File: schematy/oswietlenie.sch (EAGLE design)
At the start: 9 parts, among them U1 V_REG_317SINK

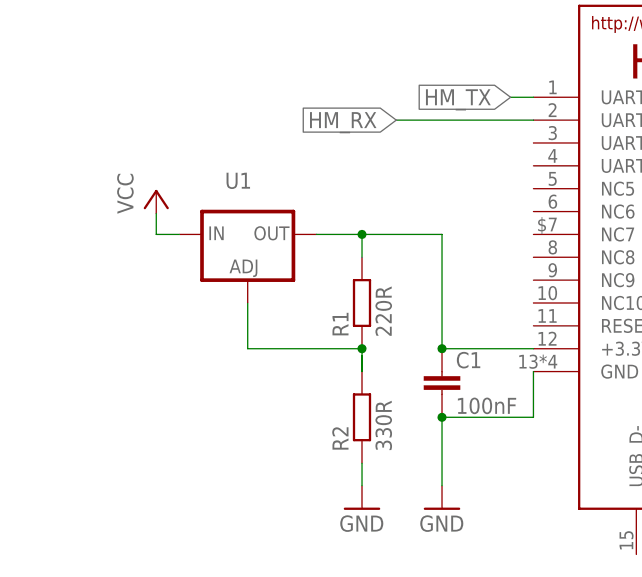
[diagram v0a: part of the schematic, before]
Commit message: update`
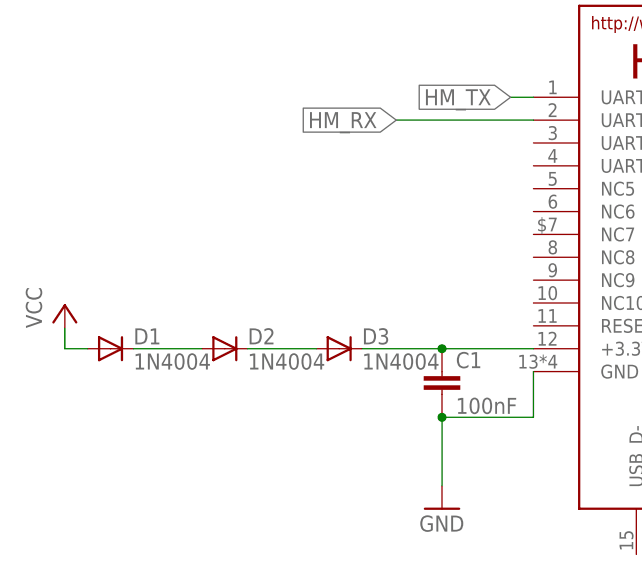
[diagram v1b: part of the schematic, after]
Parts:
- removed R1: 220R, rcl:R-EU_0204/5
- removed R2: 330R, rcl:R-EU_0204/5
- removed U1: V_REG_317SINK, SparkFun-IC-Power:V_REG_317SINK
- added D1, D2, D3: 1N4004, diode:1N4004
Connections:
- new net N$1: D1.C, D2.A
- net GND: no longer R2.1
- net N$5: now also D3.C; no longer R1.2, U1.OUT
- net N$6: now also D2.C, D3.A; no longer R1.1, R2.2, U1.ADJ
- net VCC: now also D1.A; no longer U1.IN
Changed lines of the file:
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@@
 <part name="GND5" library="supply1" library_urn="urn:adsk.eagle:library:371" deviceset="GND" device=""/>
 <part name="P+5" library="supply1" library_urn="urn:adsk.eagle:library:371" deviceset="+5V" device=""/>
-<part name="R1" library="rcl" library_urn="urn:adsk.eagle:library:334" deviceset="R-EU_" device="0204/5" package3d_urn="urn:adsk.eagle:package:23488/1" value="220R"/>
-<part name="R2" library="rcl" library_urn="urn:adsk.eagle:library:334" deviceset="R-EU_" device="0204/5" package3d_urn="urn:adsk.eagle:package:23488/1" value="330R"/>
-<part name="GND2" library="supply1" library_urn="urn:adsk.eagle:library:371" deviceset="GND" device=""/>
 <part name="~220V" library="jumper" library_urn="urn:adsk.eagle:library:252" deviceset="JP1E" device="" package3d_urn="urn:adsk.eagle:package:15455/1"/>
-<part name="U1" library="SparkFun-IC-Power" deviceset="V_REG_317" device="SINK"/>
+<part name="D1" library="diode" library_urn="urn:adsk.eagle:library:210" deviceset="1N4004" device="" package3d_urn="urn:adsk.eagle:package:43336/1"/>
+<part name="D2" library="diode" library_urn="urn:adsk.eagle:library:210" deviceset="1N4004" device="" package3d_urn="urn:adsk.eagle:package:43336/1"/>
+<part name="D3" library="diode" library_urn="urn:adsk.eagle:library:210" deviceset="1N4004" device="" package3d_urn="urn:adsk.eagle:package:43336/1"/>
 </parts>
 <sheets>
@@
 <instance part="E1" gate="G$1" x="19.05" y="78.74"/>
 <instance part="GND3" gate="1" x="3.81" y="22.86"/>
-<instance part="P+3" gate="VCC" x="-27.94" y="58.166"/>
+<instance part="P+3" gate="VCC" x="-38.1" y="45.466"/>
 <instance part="C1" gate="G$1" x="3.81" y="38.1"/>
 <instance part="U$2" gate="G$1" x="154.94" y="43.18"/>
@@
 <instance part="GND5" gate="1" x="132.08" y="66.04"/>
 <instance part="P+5" gate="1" x="142.24" y="76.2"/>
-<instance part="R1" gate="G$1" x="-5.08" y="45.72" rot="R90"/>
-<instance part="R2" gate="G$1" x="-5.08" y="33.02" rot="R90"/>
-<instance part="GND2" gate="1" x="-5.08" y="22.86"/>
 <instance part="~220V" gate="A" x="185.42" y="27.94" rot="R180"/>
-<instance part="U1" gate="G$1" x="-17.78" y="53.34"/>
+<instance part="D1" gate="1" x="-33.02" y="40.64"/>
+<instance part="D2" gate="1" x="-20.32" y="40.64"/>
+<instance part="D3" gate="1" x="-7.62" y="40.64"/>
 </instances>
 <busses>
@@
 <segment>
 <pinref part="P+3" gate="VCC" pin="VCC"/>
-<wire x1="-27.94" y1="55.626" x2="-27.94" y2="53.34" width="0.1524" layer="91"/>
-<pinref part="U1" gate="G$1" pin="IN"/>
-<wire x1="-27.94" y1="53.34" x2="-25.4" y2="53.34" width="0.1524" layer="91"/>
+<wire x1="-38.1" y1="42.926" x2="-38.1" y2="40.64" width="0.1524" layer="91"/>
+<pinref part="D1" gate="1" pin="A"/>
+<wire x1="-38.1" y1="40.64" x2="-35.56" y2="40.64" width="0.1524" layer="91"/>
 </segment>
 </net>
@@
 <wire x1="139.7" y1="68.58" x2="132.08" y2="68.58" width="0.1524" layer="91"/>
 <pinref part="JP1" gate="A" pin="2"/>
-</segment>
-<segment>
-<pinref part="R2" gate="G$1" pin="1"/>
-<pinref part="GND2" gate="1" pin="GND"/>
-<wire x1="-5.08" y1="27.94" x2="-5.08" y2="25.4" width="0.1524" layer="91"/>
 </segment>
 </net>
@@
 <net name="N$5" class="0">
 <segment>
-<pinref part="U1" gate="G$1" pin="OUT"/>
 <pinref part="C1" gate="G$1" pin="1"/>
 <pinref part="E1" gate="G$1" pin="+3.3V"/>
 <wire x1="13.97" y1="40.64" x2="3.81" y2="40.64" width="0.1524" layer="91"/>
+<pinref part="D3" gate="1" pin="C"/>
+<wire x1="-5.08" y1="40.64" x2="3.81" y2="40.64" width="0.1524" layer="91"/>
 <junction x="3.81" y="40.64"/>
-<wire x1="3.81" y1="53.34" x2="3.81" y2="40.64" width="0.1524" layer="91"/>
-<wire x1="-10.16" y1="53.34" x2="-5.08" y2="53.34" width="0.1524" layer="91"/>
-<pinref part="R1" gate="G$1" pin="2"/>
-<wire x1="-5.08" y1="53.34" x2="3.81" y2="53.34" width="0.1524" layer="91"/>
-<wire x1="-5.08" y1="50.8" x2="-5.08" y2="53.34" width="0.1524" layer="91"/>
-<junction x="-5.08" y="53.34"/>
+</segment>
+</net>
+<net name="N$1" class="0">
+<segment>
+<pinref part="D1" gate="1" pin="C"/>
+<pinref part="D2" gate="1" pin="A"/>
+<wire x1="-30.48" y1="40.64" x2="-22.86" y2="40.64" width="0.1524" layer="91"/>
 </segment>
 </net>
 <net name="N$6" class="0">
 <segment>
-<pinref part="R2" gate="G$1" pin="2"/>
-<wire x1="-5.08" y1="39.878" x2="-5.08" y2="38.1" width="0.1524" layer="91"/>
-<pinref part="R1" gate="G$1" pin="1"/>
-<wire x1="-5.08" y1="40.64" x2="-5.08" y2="38.1" width="0.1524" layer="91"/>
-<pinref part="U1" gate="G$1" pin="ADJ"/>
-<wire x1="-17.78" y1="45.72" x2="-17.78" y2="40.64" width="0.1524" layer="91"/>
-<wire x1="-17.78" y1="40.64" x2="-5.08" y2="40.64" width="0.1524" layer="91"/>
-<junction x="-5.08" y="40.64"/>
+<pinref part="D2" gate="1" pin="C"/>
+<pinref part="D3" gate="1" pin="A"/>
+<wire x1="-17.78" y1="40.64" x2="-10.16" y2="40.64" width="0.1524" layer="91"/>
 </segment>
 </net>
